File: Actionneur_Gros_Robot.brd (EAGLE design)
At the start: 92 x 38 mm, 43 parts, among them IC1 MCP2515-I_P, M1 ARDUINO-NANO-3.0, M10 SERVO, M11 SERVO, M2 SERVO, M3 SERVO, M4 SERVO, M5 SERVO, M6 SERVO, M7 SERVO, M8 SERVO, M9 SERVO, Y1 16MHz

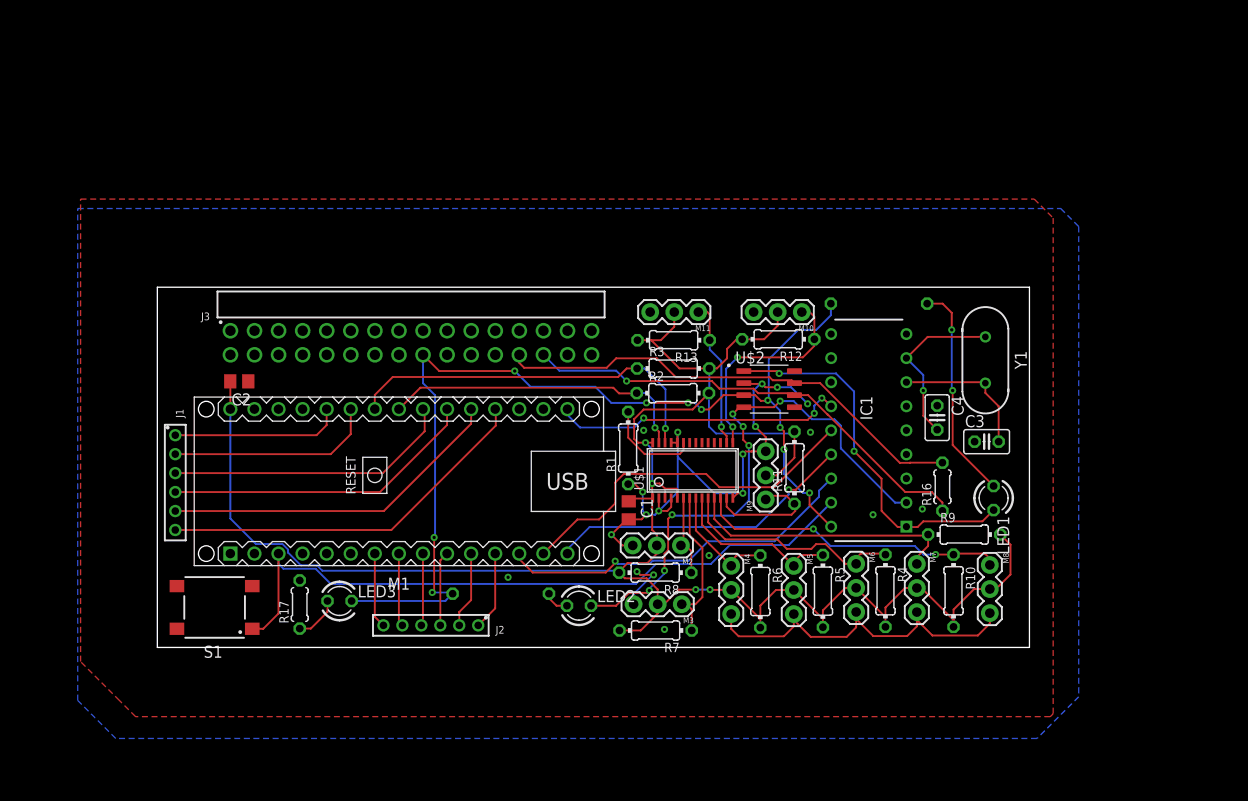
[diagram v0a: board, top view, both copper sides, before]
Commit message: v2 en cours de révision
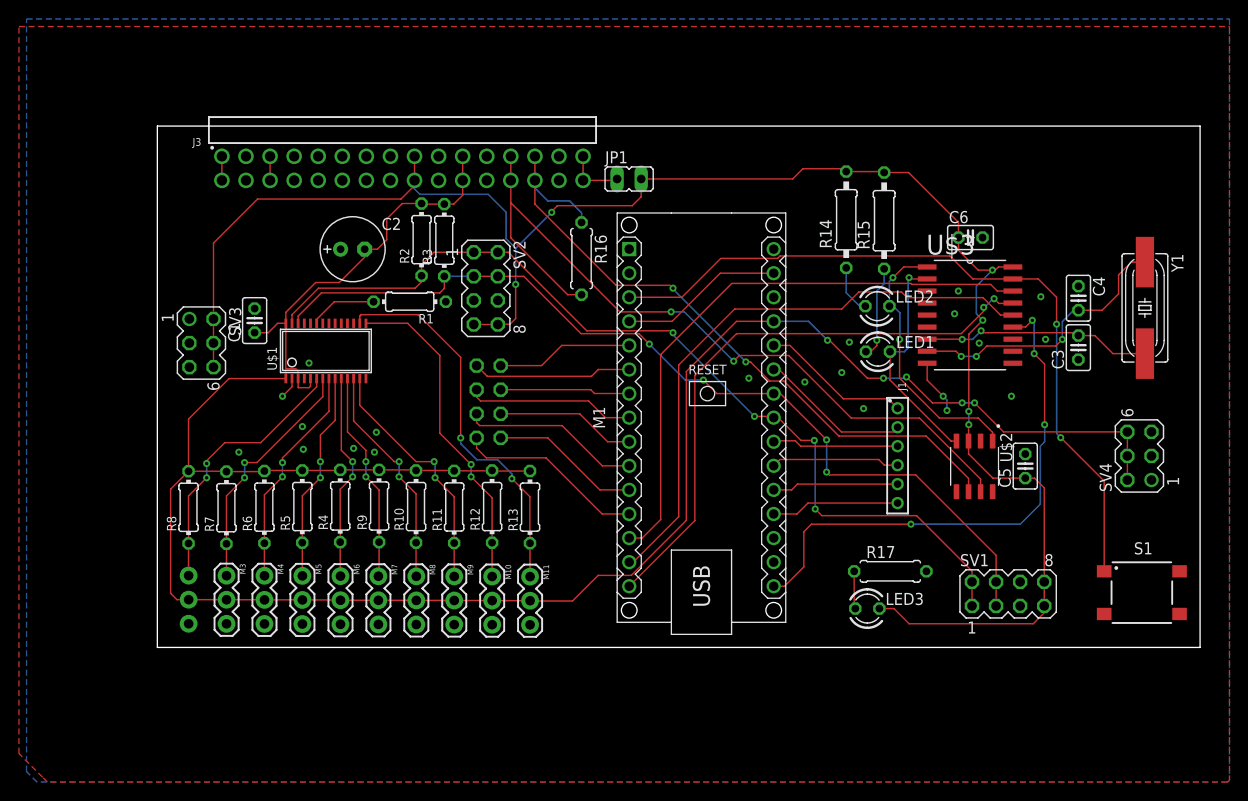
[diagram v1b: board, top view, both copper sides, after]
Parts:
- removed IC1: MCP2515-I_P, MCP2515-I_P:DIP794W56P254L2286H533Q18N
- added C5, C6: 100nF, rcl:C025-025X050
- added JP1: (no value), jumper:JP1
- added SV1, SV2: (no value), con-lstb:MA04-2
- added SV3, SV4: (no value), con-lstb:MA03-2
- added U$3: MCP2515T-E/SO, MCP2515-I_P:SOIC127P1030X265-18N
- C1: value (none) -> 100nF; device rcl:C0805 -> rcl:C025-025X050
- C2: value (none) -> 10uF; device rcl:C0805 -> rcl:E2,5-7
- C3, C4: value (none) -> 22pF
- J2: device Wurth_Connectors_WR-PHD:62000611121 -> con-lstb:MA04-2
- R14, R15: value (none) -> 680R
- R16, R17: device ___RCL:0204/5 -> rcl:0207/7
- Y1: device Wurth_Quartz Crystals & Oscillators_WE-XTAL:WE-XTAL_HC49 -> crystal:HC49UP
- moved S1 97.8 mm to (103.9, 5.78), turned to 0 degrees
- moved J1 76.3 mm to (78.1, 20.2)
- moved R17 62.4 mm to (77.3, 8.03), turned to 0 degrees
- moved R9 61.8 mm to (23.4, 14.9), turned to 90 degrees
- moved M8 60.5 mm to (27.3, 7.50)
- moved R4 58.2 mm to (19.3, 14.9), turned to 90 degrees
- moved R10 57.4 mm to (27.3, 14.9), turned to 90 degrees
- moved M7 56.8 mm to (23.3, 7.51)
- moved LED3 55.7 mm to (74.9, 4.10)
- moved R5 55.6 mm to (15.3, 14.9), turned to 90 degrees
- moved M6 54.4 mm to (19.3, 7.52)
- moved R14 53.7 mm to (72.7, 45.1), flipped to the top, turned to 90 degrees
- moved R6 53.1 mm to (11.3, 14.8), turned to 90 degrees
- moved M2 52.0 mm to (3.30, 7.58), flipped to the bottom, turned to 270 degrees
- moved M5 51.9 mm to (15.3, 7.55)
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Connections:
- removed net 5V: M1.J2.4
- removed net N$15: C4.2, IC1.8, Y1.1
- new net +12V: J3.1, J3.2
- new net N$21: C4.2, U$3.8, Y1.1
- new net N$24: C3.2, U$3.7, Y1.2
- new net VIN: M1.J2.1
- net BAU: now also J3.31, JP1.1
- net CANH: now also J3.25
- net CANL: now also J3.27
- net CHIP_SELECT: now also U$3.16; no longer IC1.16
- net GND: now also C2.+, C5.2, C6.2, J3.11, J3.12, J3.19, J3.23, J3.24, J3.3, J3.4, J3.7, J3.8, S1.2, SV1.5, SV1.6, SV2.5, SV2.6, SV3.1, SV3.3, SV3.5, SV4.1, SV4.3, SV4.5, U$3.9; no longer C2.1, IC1.9
- net I2C_SCL: now also SV1.3, SV1.4, SV2.3, SV2.4
- net I2C_SDA: now also SV1.1, SV1.2, SV2.1, SV2.2
- net IRQ0: now also J2.1
- net IRQ1: now also J2.2
- net MISO1: now also U$3.15; no longer IC1.15
- net MOSI1: now also U$3.14; no longer IC1.14
- net N$10: now also J2.6; no longer J2.3
- net N$11: now also J2.5; no longer J2.4
- net N$12: now also J2.4; no longer J2.5
- net N$13: now also J2.3; no longer J2.6
- net N$14: now also J3.5, J3.6; no longer C3.2, IC1.7, Y1.2
- net N$8: now also J2.8; no longer J2.1
- net N$9: now also J2.7; no longer J2.2
- net RESET: now also U$3.17; no longer IC1.17
- net RX_CAN1: now also LED1.K, U$3.2; no longer IC1.2, LED2.K
- net SCK1: now also U$3.13; no longer IC1.13
- net TX_CAN1: now also LED2.K, U$3.1; no longer IC1.1, LED1.K
- net VCC: now also C2.-, J3.21, J3.22, M1.J2.4, SV4.2, SV4.4, SV4.6; no longer C2.2, M1.J2.1
- net VDD: now also C5.1, C6.1, J3.17, JP1.2, SV1.7, SV1.8, SV2.7, SV2.8, SV3.2, SV3.4, SV3.6, U$3.18; no longer IC1.18
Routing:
- net VDD: track 109.3 -> 193.4 mm, vias 10 -> 6
- net GND: track 104.6 -> 25.5 mm, vias 20 -> 21
- net I2C_SDA: track 33.1 -> 98.3 mm, vias 1 -> 4
- net I2C_SCL: track 39.9 -> 96.4 mm, vias 1 -> 4
- net RX_CAN1: track 59.2 -> 24.2 mm, vias 7 -> 1
- net VCC: track 214.2 -> 246.5 mm, vias 4 -> 5
- net CANH: track 50.7 -> 82.0 mm, vias 0 -> 2
- net MISO1: track 32.7 -> 62.5 mm, vias 1 -> 2
- net N$21: track 0.00 -> 29.6 mm, vias 0 -> 3
- net N$2: track 40.1 -> 13.5 mm
- net SERVO_9: track 15.6 -> 40.8 mm, vias 1 -> 2
- net SCK1: track 31.3 -> 56.3 mm, vias 3 -> 4
- net MOSI1: track 38.2 -> 62.7 mm
- net N$24: track 0.00 -> 24.4 mm, vias 0 -> 2
- net N$3: track 36.6 -> 13.3 mm
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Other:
- board size 92 x 38 mm -> 110 x 55 mm
